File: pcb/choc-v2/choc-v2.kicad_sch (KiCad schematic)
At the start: 139 parts, among them J1 OLED, J2 Conn_01x02_Female, J3 Conn_01x03_Female, SW1 SW_Push, SW2 RotaryEncoder_Switch, SW3 RotaryEncoder_Switch, SW4 SW_SPDT, U1 Elite-C

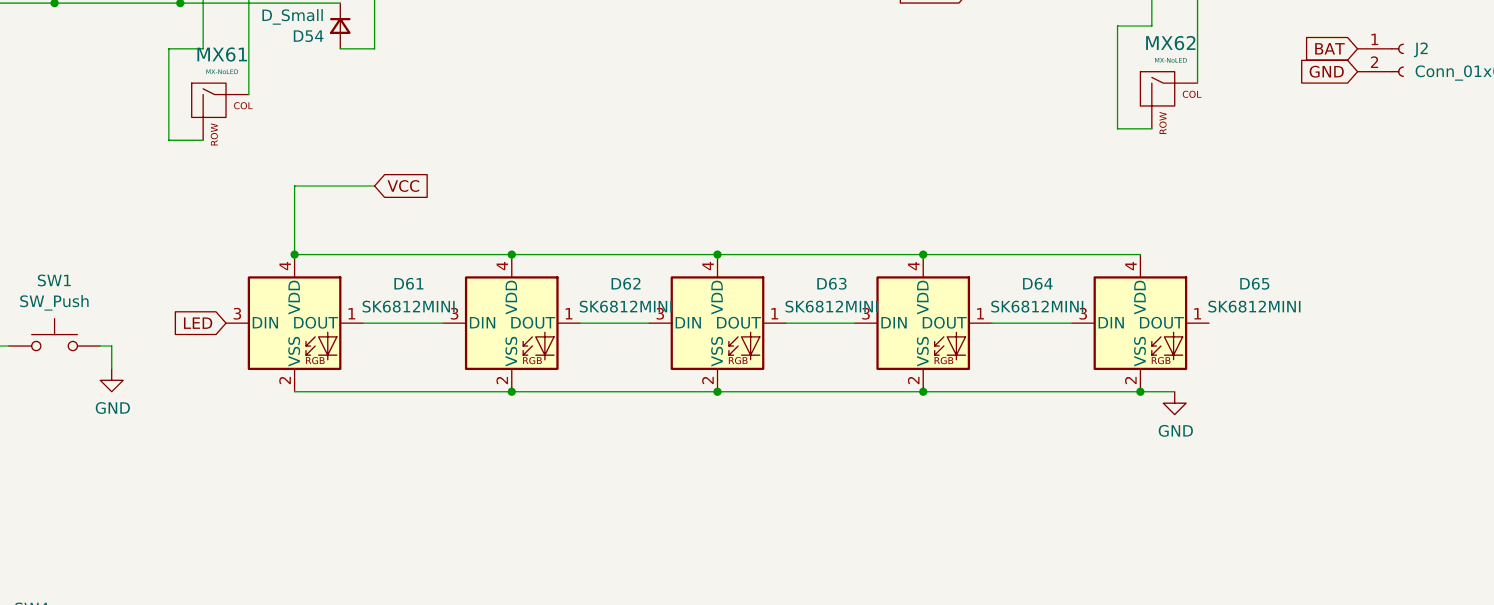
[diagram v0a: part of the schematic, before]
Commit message: Checkpoint commit.
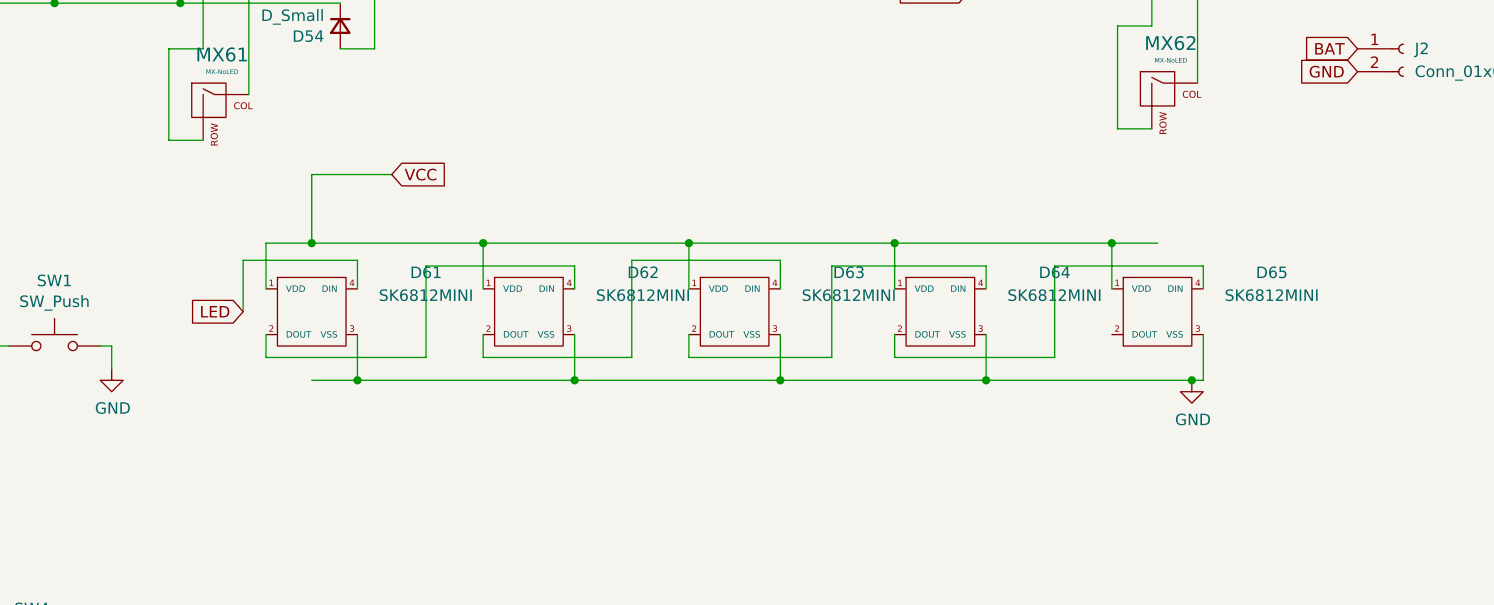
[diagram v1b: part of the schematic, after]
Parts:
- removed D61, D62, D63, D64, D65: SK6812MINI, footprints:YS-SK6812MINI-E, symbol LED:SK6812MINI
- added D61, D62, D63, D64, D65: SK6812MINI, footprints:YS-SK6812MINI-E, symbol atreyu-pcb2:SK6812MINI_LED
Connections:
- net GND: now also D61.3 (VSS), D62.3 (VSS), D63.3 (VSS), D64.3 (VSS), D65.3 (VSS)
- net LED: now also D61.4 (DIN)
- net VCC: now also D61.1 (VDD), D62.1 (VDD), D63.1 (VDD), D64.1 (VDD), D65.1 (VDD)
- new net: D62.2 (DOUT), D63.4 (DIN)
- new net: D61.2 (DOUT), D62.4 (DIN)
- new net: D64.2 (DOUT), D65.4 (DIN)
- new net: D63.2 (DOUT), D64.4 (DIN)
